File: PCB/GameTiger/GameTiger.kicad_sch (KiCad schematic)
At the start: 77 parts, among them J1 USB TypeC Connector, J2 503398-1892, J3 LCD Display, J4 Speaker, Q3 DMG3415, U1 RP2040, U2 MCP73831-2-OT, U3 W25Q128JVSIQ, U4 PAM8302A, U5 AP2112K-3.3, U6 PCF8574TS, Y1 12MHZ XTal

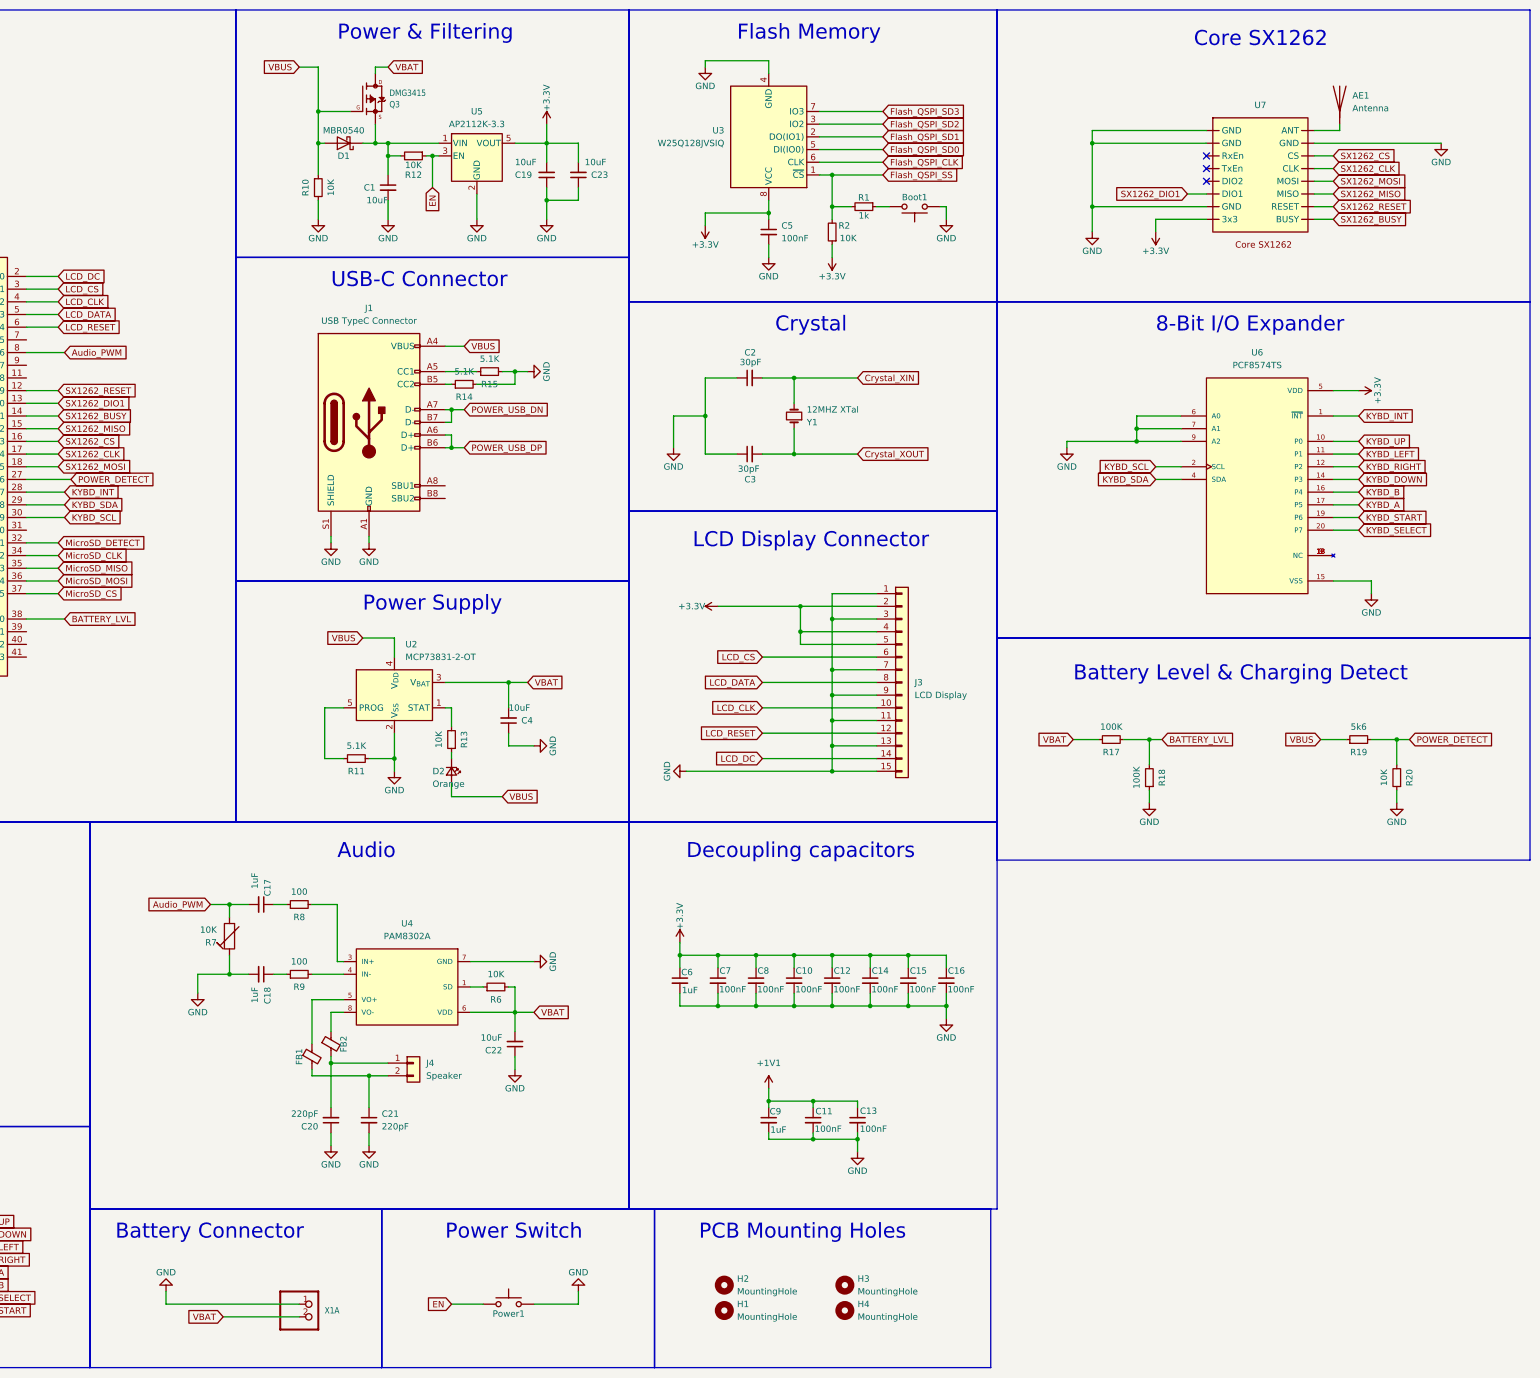
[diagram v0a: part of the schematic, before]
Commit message: Completed updating the PCB design for peer review
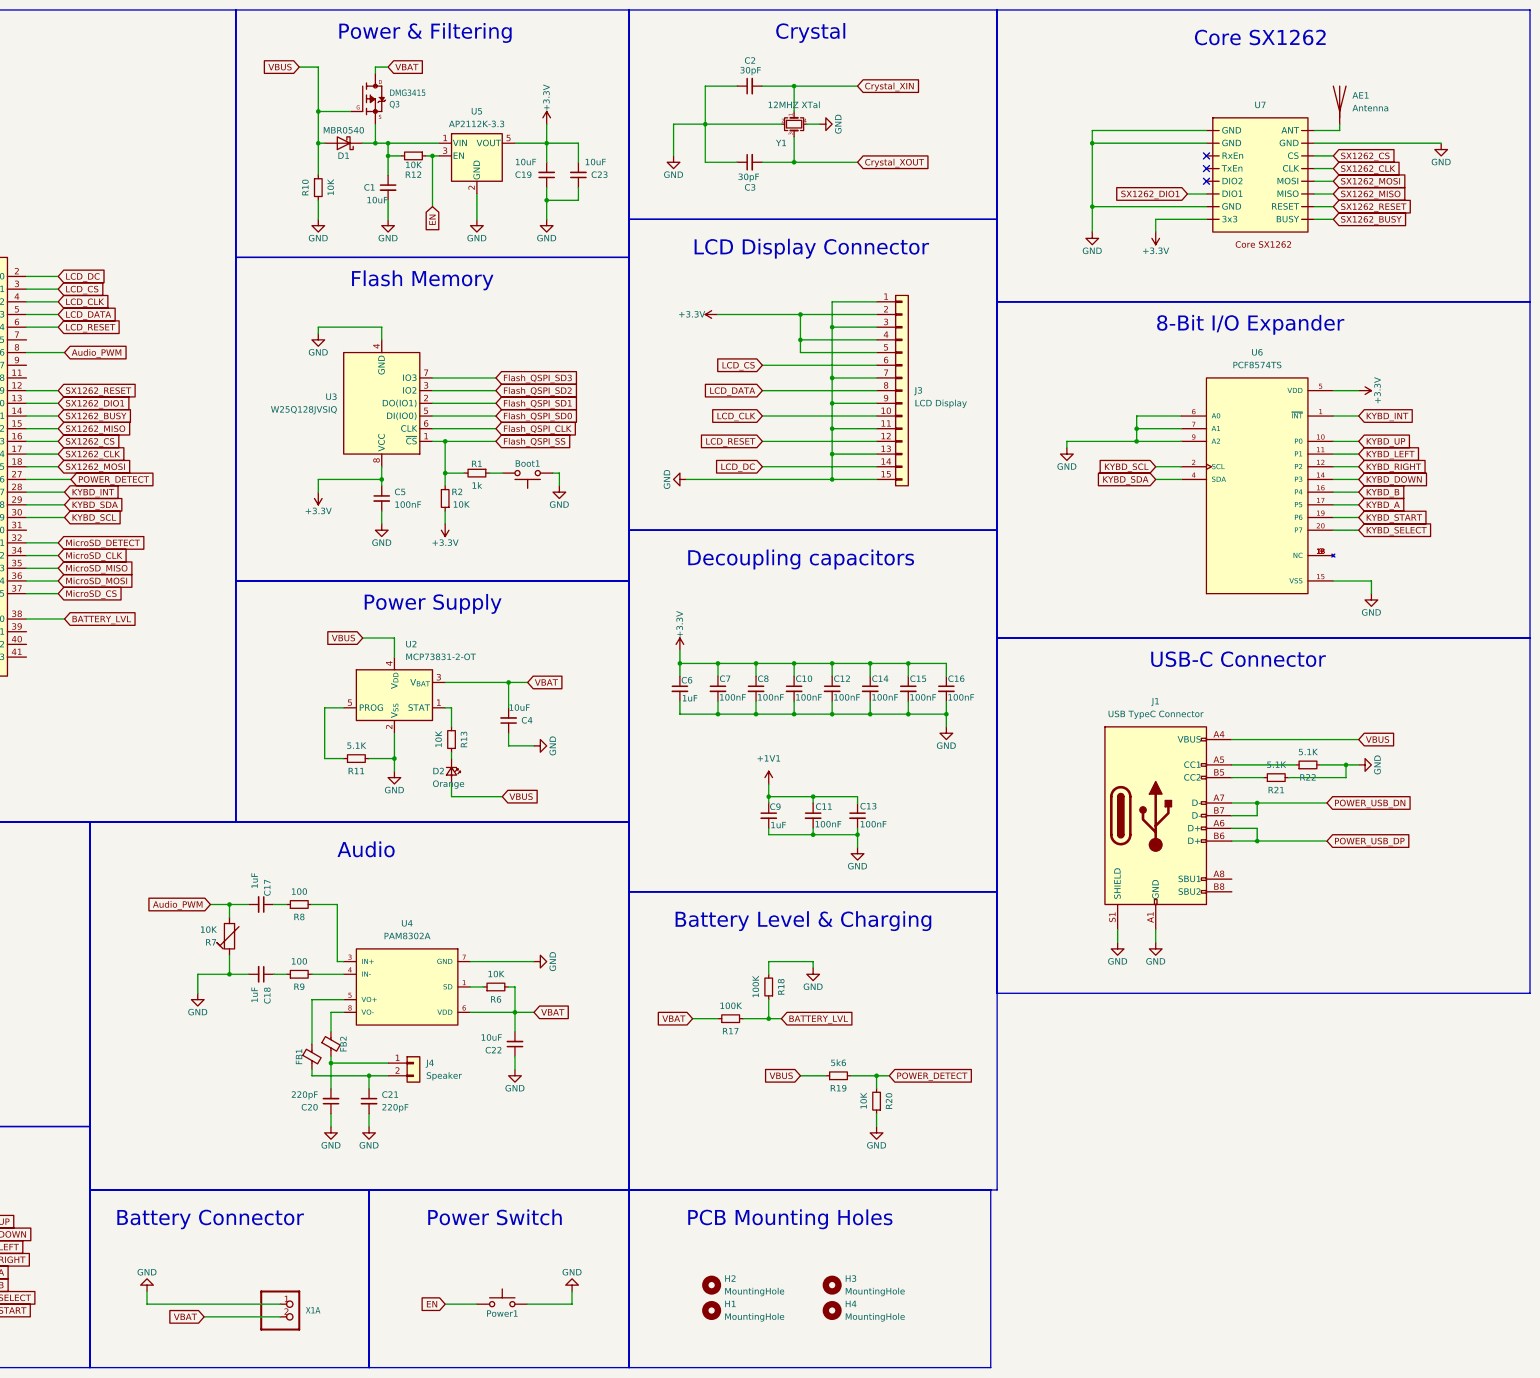
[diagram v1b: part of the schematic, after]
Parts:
- removed R14, R15: 5.1K, Resistor_SMD:R_0402_1005Metric, symbol Device:R_Small
- removed Y1: 12MHZ XTal, Crystal:Crystal_SMD_3225-4Pin_3.2x2.5mm, symbol Device:Crystal_Small
- added R21, R22: 5.1K, Resistor_SMD:R_0402_1005Metric, symbol Device:R_Small
- added Y1: 12MHZ XTal, Crystal:Crystal_SMD_3225-4Pin_3.2x2.5mm, symbol Device:Crystal_GND24_Small
- A1, B1, Down1, Left1, Right1, Up1: footprint Button_Switch_SMD:SW_Push_1P1T_NO_CK_PTS125Sx43PSMTR -> Button_Switch_THT:SW_PUSH-12mm; Manufacturer C&K -> (none); Mfr.Part # PTS125SJM73PSMTR2LFS -> (none); Mouser (none) -> 653-B3F-1052; Size SMD,12x12mm -> (none)
- AE1: footprint Connector_Pin:Pin_D1.0mm_L10.0mm -> Connector_Pin:Pin_D1.0mm_L10.0mm_LooseFit
- Boot1, Reset1: Mouser (none) -> 653-B3U-1000P
- C1, C19, C22, C23, C4: Mouser (none) -> 187-CL21A106KAFN3NE; Size 0805_2012Metric -> (none)
- C10, C11, C12, C13, C14, C15, C16, C5, C7, C8: Mouser (none) -> 187-CL05A104KO5NNWC; Size 0402_1005Metric -> (none)
- C17, C18, C6, C9: Mouser (none) -> 187-CL05A105KP5NNWC; Size 0402_1005Metric -> (none)
- C2, C3: Material C0G -> (none); Size 0402_1005Metric -> (none); Tolerance 5% -> (none); Voltage 50v -> (none)
- C20, C21: Mouser (none) -> 187-CL21C221JB61PNL; Size 0805_2012Metric -> (none)
- D1: Mouser (none) -> 512-MBR0540
- D2: Mouser (none) -> 78-VLMO1500-GS08
- FB1, FB2: LCSC C44838 -> C85835; Manuf. Part # CBW201209U102T -> BLM21BD102SN1D; Manufacturer FH (Guangdong Fenghua Advanced Tech) -> Murata Electronics; Mouser (none) -> 81-BLM21B102S; Size 0805 -> (none)
- J1: LCSC C165948 -> C2988369; Manuf. Part # TYPE-C-31-M-12 -> GT-USB-7010ASV; Manufacturer Korean Hroparts Elec -> JAE Electronics; Mouser (none) -> 656-DX07S016JA1R1500
- J2: Mouser (none) -> 538-503398-1892
- J3: LCSC C262664 -> C262209; Manuf. Part # AFC01-S15FCA-00 -> 1-1734839-5; Manufacturer JUSHUO -> (none); Mouser (none) -> 571-1-1734839-5; Size SMD,P=0.5mm -> (none)
- Power1: Mouser (none) -> 611-JS102011SAQN; Size SMD -> (none)
- Q3: Mouser (none) -> 621-DMG3415U-7
- R1, R5: Mouser (none) -> 71-CRCW04021K00FKEDC; Power 63mW -> (none); Size 0402_1005Metric -> (none)
- R10, R12, R13, R16, R2, R6: Mouser (none) -> 71-CRCW040210K0FKEDC; Power 63mW -> (none); Size 0402_1005Metric -> (none)
- R11: Mouser (none) -> 71-CRCW04025K10FKEDC; Power 63mW -> (none); Size 0402_1005Metric -> (none)
- R17, R18: footprint Resistor_SMD:R_0603_1608Metric -> Resistor_SMD:R_0402_1005Metric; LCSC C25803 -> C25741; Mouser (none) -> 71-CRCW0402100KFKEDC; Size 0603_1608Metric -> (none)
- R19: footprint Resistor_SMD:R_0603_1608Metric -> Resistor_SMD:R_0402_1005Metric; LCSC (none) -> C25908; Mouser (none) -> 71-CRCW04025K60FKEDC; Size 0603_1608Metric -> (none)
- R20: footprint Resistor_SMD:R_0603_1608Metric -> Resistor_SMD:R_0402_1005Metric; LCSC (none) -> C25744; Mouser (none) -> 71-CRCW040210K0FKEDC; Size 0603_1608Metric -> (none)
- R3, R4: footprint Resistor_SMD:R_0603_1608Metric -> Resistor_SMD:R_0402_1005Metric; Mouser (none) -> 71-CRCW040227R0FKEDC; Power 63mW -> (none); Size 0603_1608Metric -> (none)
- R7: Mouser (none) -> 652-TC33X-2-103E
- R8, R9: Mouser (none) -> 71-CRCW0402100RFKEDC; Power 63mW -> (none); Size 0402_1005Metric -> (none)
- Select1, Start1: footprint Button_Switch_SMD:SW_SPST_Omron_B3FS-105xP -> Button_Switch_THT:SW_TH_Tactile_Omron_B3F-10xx; LCSC C306879 -> C411882; Manufacturer Omron Electronics -> (none); Mfr.Part # B3FS-1052P -> (none); Mouser (none) -> 653-B3F-1052; Size SMD -> SMD,6x6mm
- U1: Mouser (none) -> 358-SC091413
- U2: Mouser (none) -> 579-MCP73831T-2ACIOT
- U3: Mouser (none) -> 454-W25Q128JVSIQ
- U4: Mouser (none) -> 621-PAM8302AASCR
- U5: Mouser (none) -> 621-AP2112K-3.3TRG1
- U6: Manuf. Part # PCF8574TS -> PCF8574TS/3,118; Mouser (none) -> 771-PCF8574TDK-T
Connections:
- net BATTERY_LVL: now also R18.1; no longer R18.2
- net Crystal_XIN: now also Y1.1
- net Crystal_XOUT: now also Y1.3
- net GND: now also R18.2, R21.2, R22.2, Y1.2, Y1.4; no longer R18.1
- net at J1.B5 (CC2): now also R21.1
- net at J1.A5 (CC1): now also R22.1
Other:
- note added: "Battery Level & Charging"
- note removed: "Battery Level & Charging Detect"
- moved on the sheet: Boot1, C10, C11, C12, C13, C14, C15, C16, C2, C20, C21, C3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
